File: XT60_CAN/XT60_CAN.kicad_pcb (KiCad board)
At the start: 2 copper layers, 41 parts, among them J1 XT60_IN, J15 XT60_CH4, J16 XT60_CH5, J19 +5V, J2 XT60_CH1, J20 +5V, J3 +9V, J4 +12V, J5 +9V, J6 +12V, J8 XT60_CH2, J9 XT60_CH3, U1 MP1584, U2 MP1584, U3 MP1584

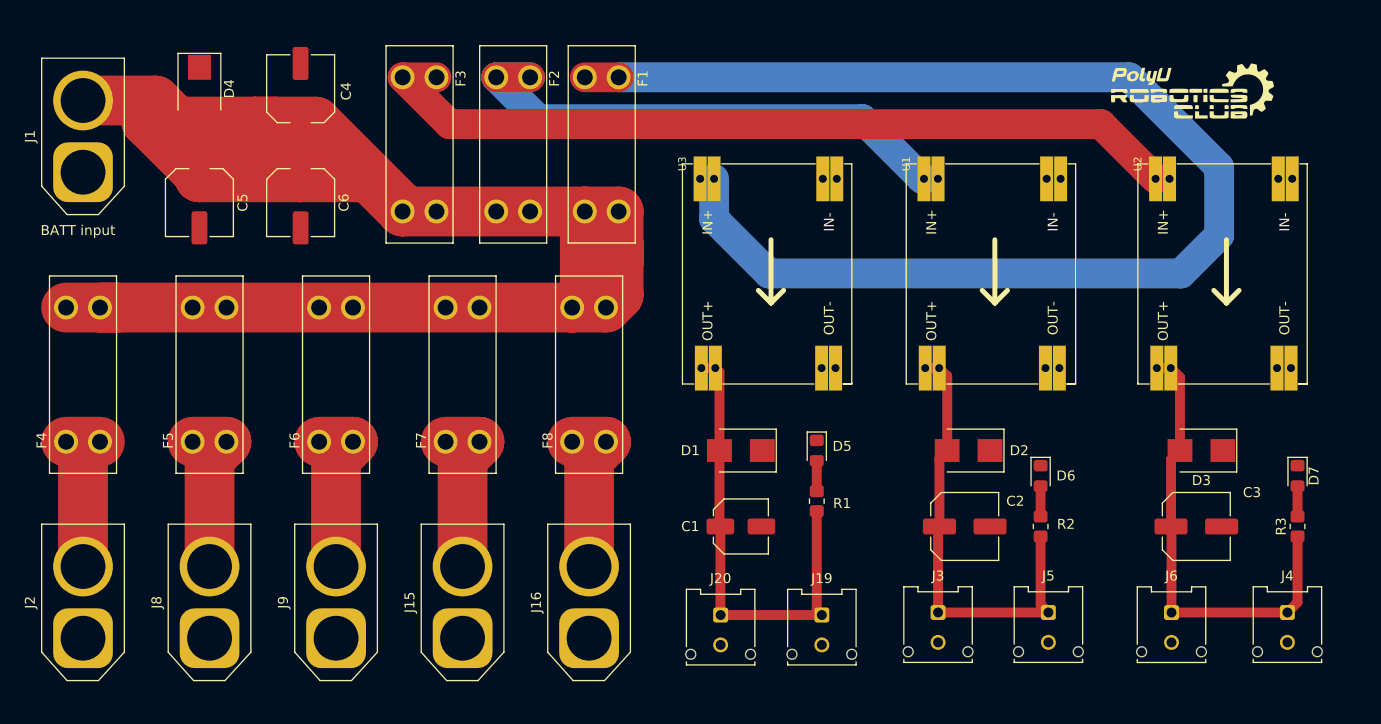
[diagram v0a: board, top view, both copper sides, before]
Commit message: power_board
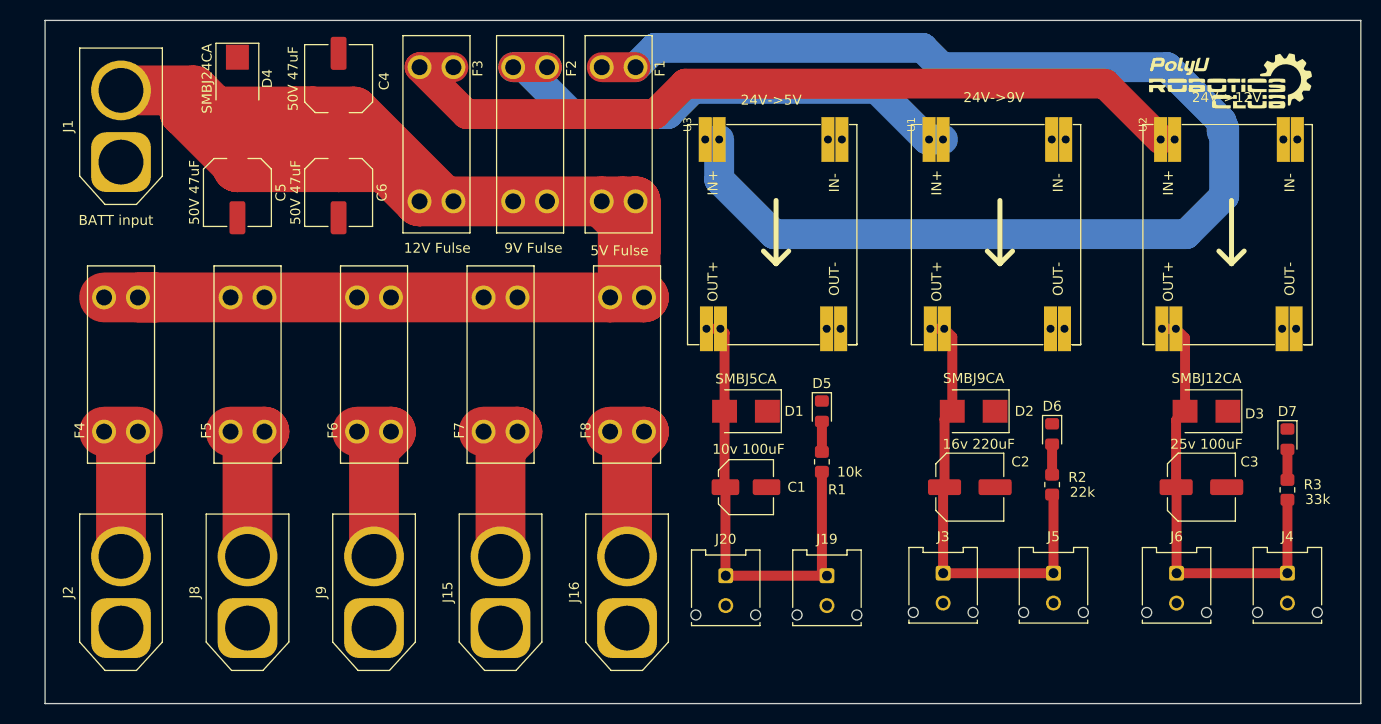
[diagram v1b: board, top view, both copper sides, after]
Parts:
- removed the G*** at (90.9, 49.3)
- moved D6 4.36 mm to (159.5, 64.4)
- moved R2 4.36 mm to (159.5, 69.5)
- moved D2 3.98 mm to (151.6, 62.1)
- moved D3 3.98 mm to (175.0, 62.1)
- moved D5 3.98 mm to (136.4, 62.1)
- moved J19 3.98 mm to (136.9, 78.6)
- moved J20 3.98 mm to (126.7, 78.6)
- moved J3 3.98 mm to (148.6, 78.3)
- moved J5 3.98 mm to (159.7, 78.3)
- moved J6 3.98 mm to (172.0, 78.4)
- moved R1 3.98 mm to (136.4, 67.2)
- moved C1 3.98 mm to (128.8, 69.7)
- moved C2 3.98 mm to (151.3, 69.7)
- moved C3 3.98 mm to (174.5, 69.7)
- moved D1 3.98 mm to (128.8, 62.1)
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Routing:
- net +24V: track 202.5 -> 199.8 mm
- net +12V: track 46.4 -> 45.2 mm
- net Net-(F2-Pad1): track 54.0 -> 53.4 mm
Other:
- board outline added: 132.1 x 68.6 mm
- board text added: "10k"
- board text added: "10v 100uF"
- board text added: "12V Fulse"
- board text added: "16v 220uF"
- board text added: "22k"
- board text added: "24V->12V"
- board text added: "24V->5V"
- board text added: "24V->9V"
- board text added: "25v 100uF"
- board text added: "33k"
- board text added: "50V 47uF"
- board text added: "5V Fulse"
- board text added: "9V Fulse"
- board text added: "SMBJ12CA"
- board text added: "SMBJ24CA"
- board text added: "SMBJ5CA"
- board text added: "SMBJ9CA"
